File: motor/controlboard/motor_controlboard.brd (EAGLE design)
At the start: 47 x 70.8 mm, 27 parts, among them IC1 74AHC1G32DCK

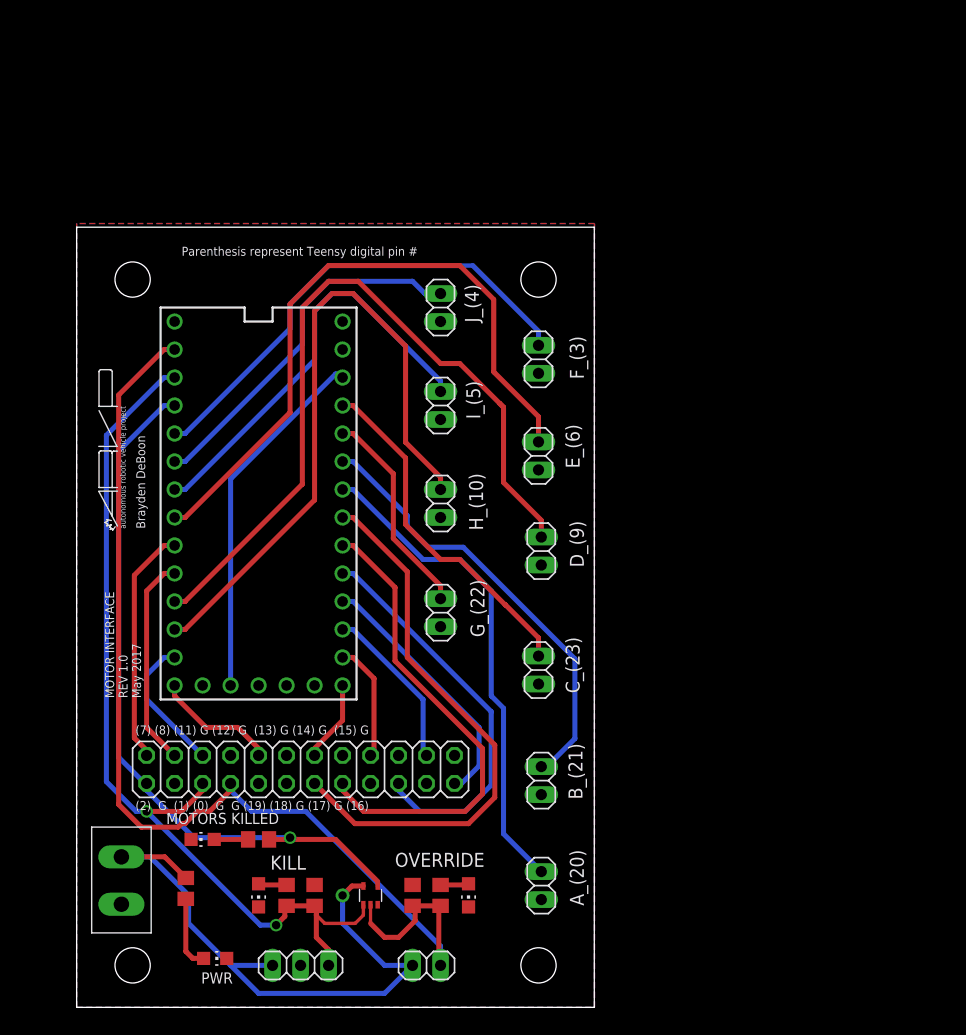
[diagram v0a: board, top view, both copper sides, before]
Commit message: Updated board May 28
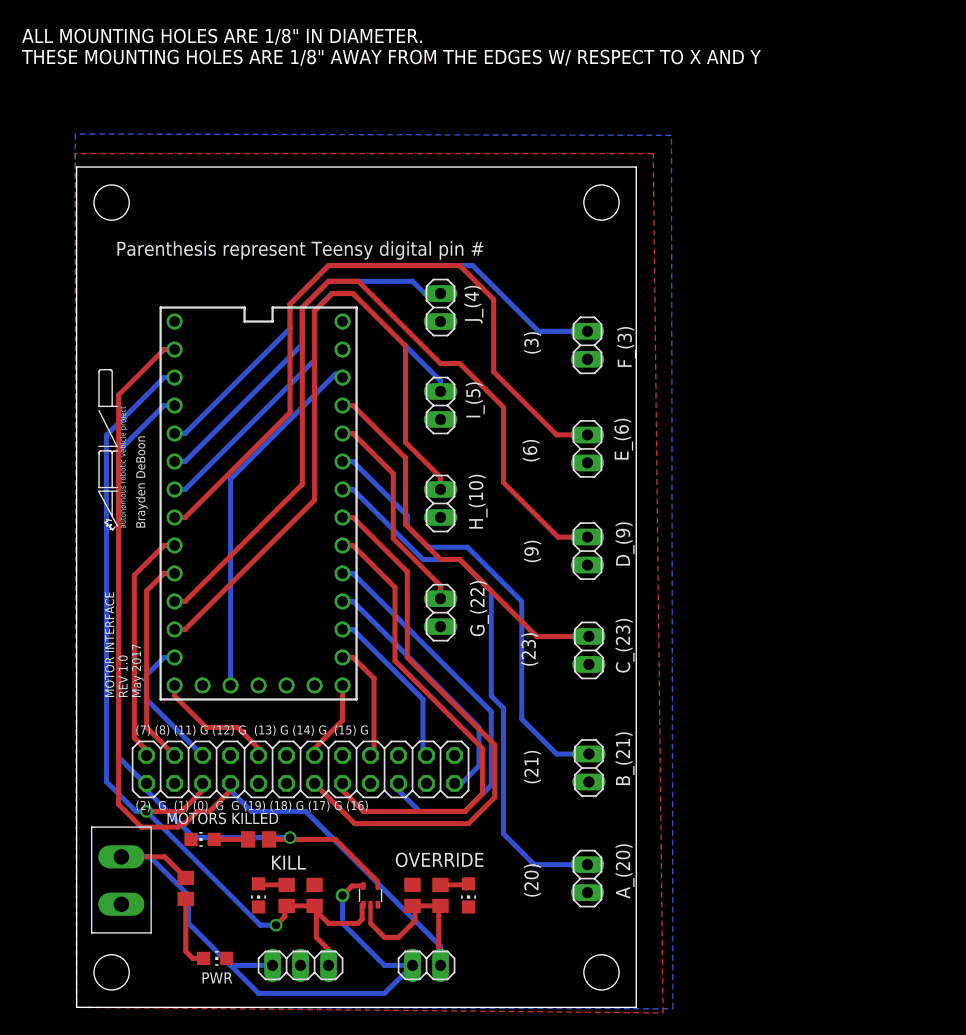
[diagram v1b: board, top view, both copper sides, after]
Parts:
- moved C_(23) 4.91 mm to (46.5, 32.4)
- moved F_(3) 4.62 mm to (46.4, 60.1)
- moved E_(6) 4.49 mm to (46.4, 50.7)
- moved B_(21) 4.47 mm to (46.5, 21.7)
- moved A_(20) 4.24 mm to (46.4, 11.7)
- moved D_(9) 4.19 mm to (46.4, 41.4)
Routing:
- net SIG_10: track 44.7 -> 48.6 mm
- net SIG_1: track 44.4 -> 47.6 mm
- net SIG_7: track 31.7 -> 34.6 mm
- net SIG_4: track 60.1 -> 62.9 mm
- net SIG_5: track 69.7 -> 72.5 mm
- net KILL: track 83.5 -> 84.4 mm
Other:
- board size 47 x 70.8 mm -> 50.8 x 76.3 mm
- board text added: "(20)"
- board text added: "(21)"
- board text added: "(23)"
- board text added: "(3)"
- board text added: "(6)"
- board text added: "(9)"
- board text added: "ALL MOUNTING HOLES ARE 1/8" IN DIAMETER. THESE MOUNTING HOLES ARE 1/8" AWAY FROM THE EDGES W/ RESPECT TO X AND Y"
